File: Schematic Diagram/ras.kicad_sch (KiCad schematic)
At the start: 2 parts

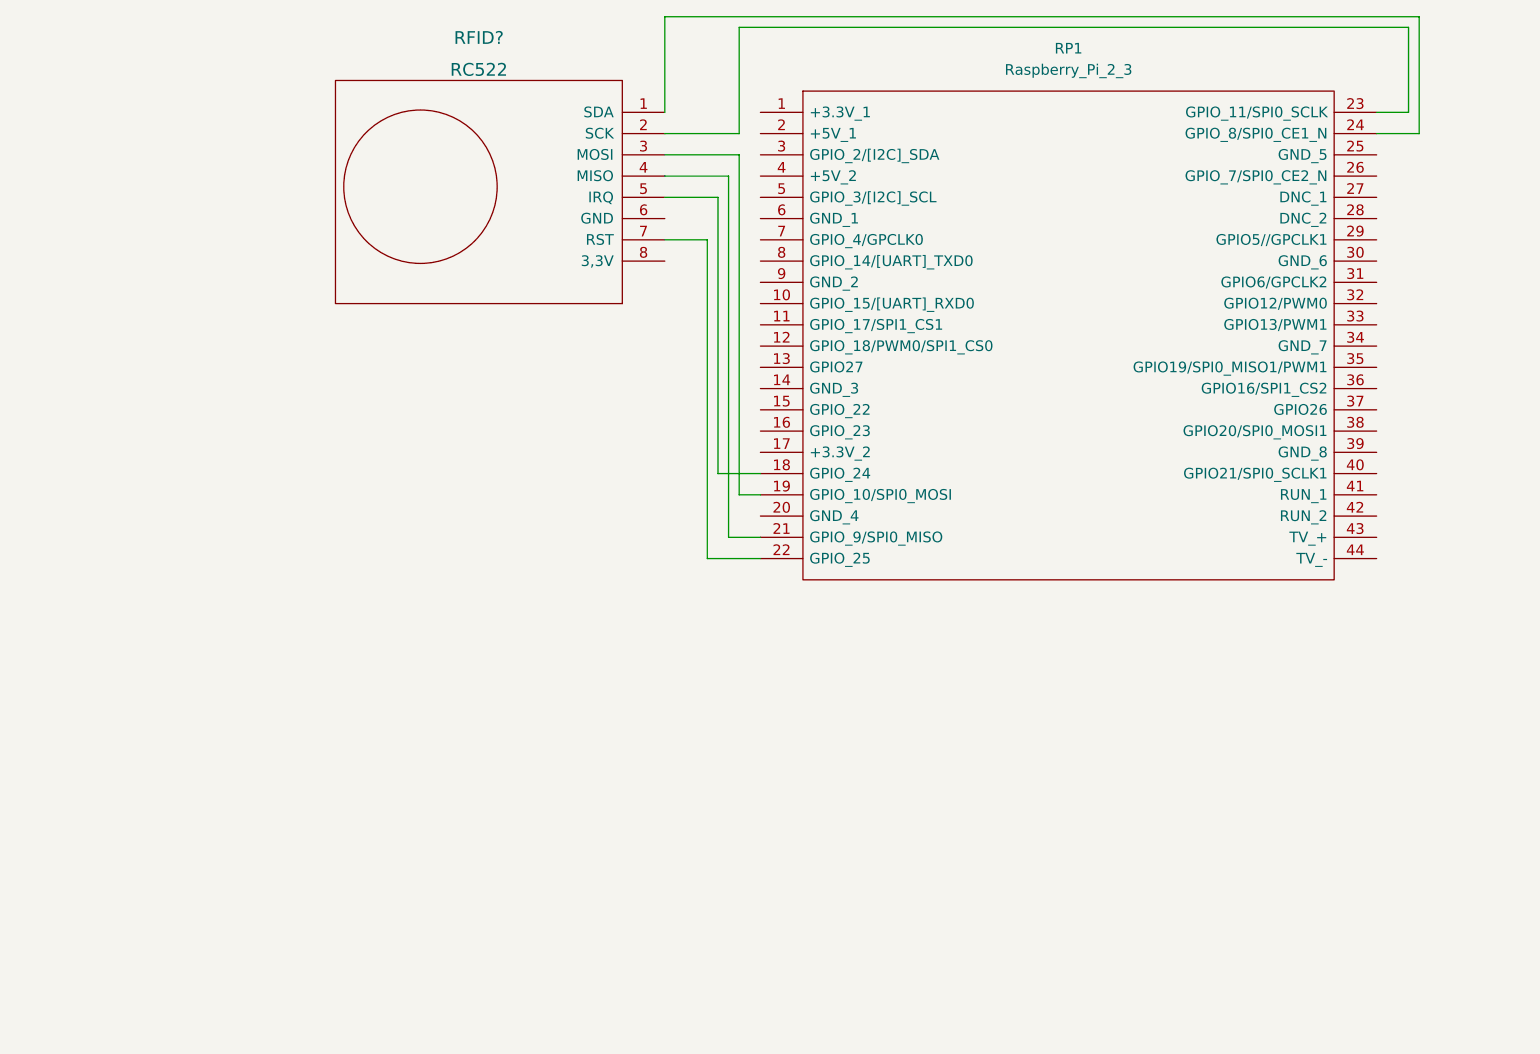
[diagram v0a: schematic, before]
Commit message: put RC522
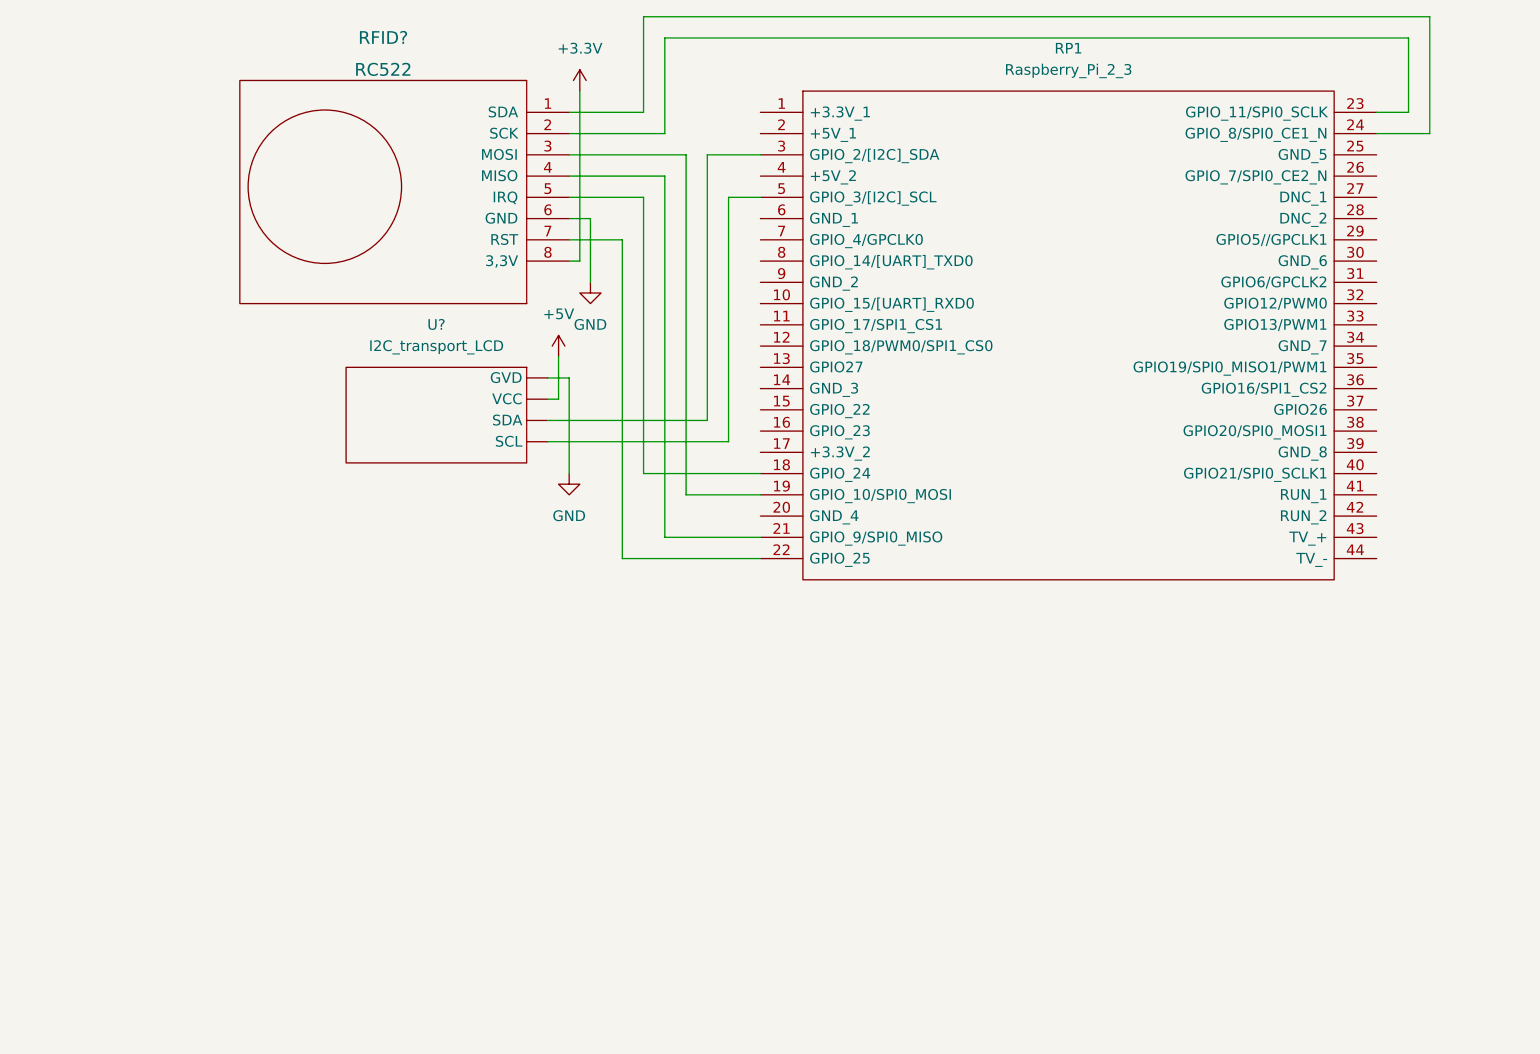
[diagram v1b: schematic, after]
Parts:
- added U?: I2C_transport_LCD, symbol project:I2C_transport_LCD
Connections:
- net at RP1.3 (GPIO_2/[I2C]_SDA): now also U?. (VCC)
- net at RP1.5 (GPIO_3/[I2C]_SCL): now also U?. (VCC)
- net GND: now reaches RFID?.6 (GND)
- net GND: now also U?. (VCC)
- net +3V3: now reaches RFID?.8 (3,3V)
- new net +5V: U?. (VCC)
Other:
- moved on the sheet: RFID?

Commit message: put LED
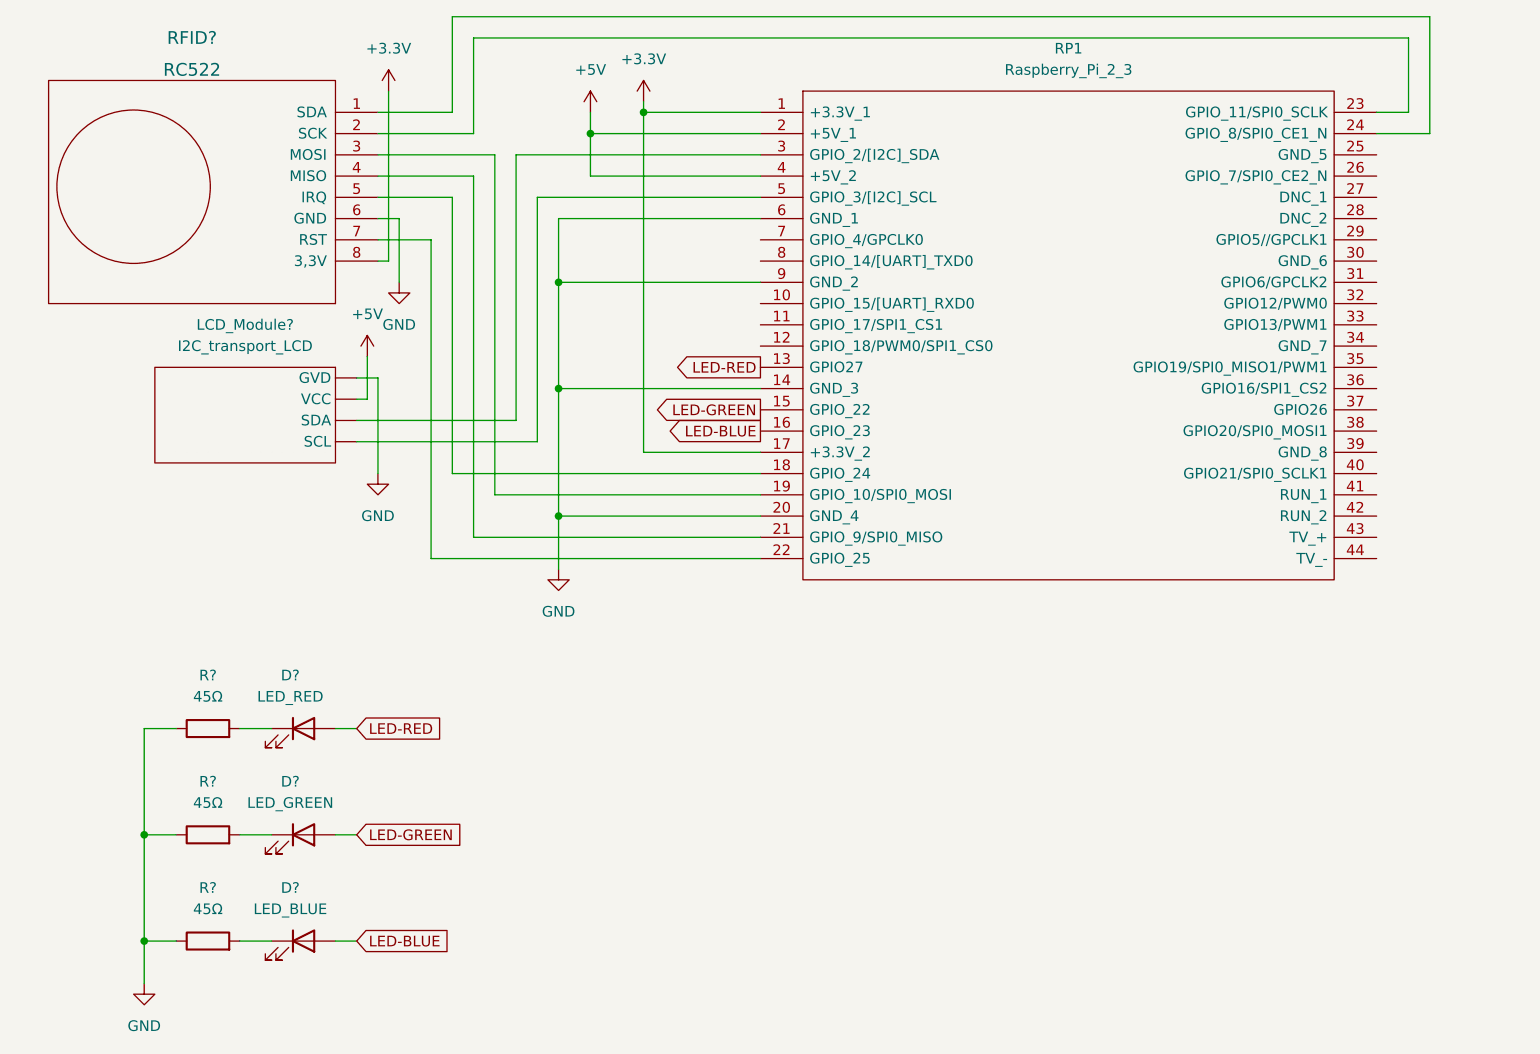
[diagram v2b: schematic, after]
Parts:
- removed U?: I2C_transport_LCD, symbol project:I2C_transport_LCD
- added D?: LED_RED, symbol Device:LED
- added D?: LED_GREEN, symbol Device:LED
- added D?: LED_BLUE, symbol Device:LED
- added LCD_Module?: I2C_transport_LCD, symbol project:I2C_transport_LCD
- added R? (x3): 45Ω, symbol Device:R
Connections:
- net +3V3: now also RP1.1 (+3.3V_1), RP1.17 (+3.3V_2)
- net +5V: now also RP1.2 (+5V_1), RP1.4 (+5V_2), LCD_Module?. (VCC)
- net GND: now also RP1.14 (GND_3), RP1.20 (GND_4), RP1.6 (GND_1), RP1.9 (GND_2), LCD_Module?. (VCC), R?.1, R?.1, R?.1
- net LED-RED: now reaches RP1.13 (GPIO27)
- net LED-RED: now also D?.2 (A)
- net LED-GREEN: now reaches RP1.15 (GPIO_22)
- net LED-GREEN: now also D?.2 (A)
- net LED-BLUE: now reaches RP1.16 (GPIO_23)
- net LED-BLUE: now also D?.2 (A)
- net at RP1.3 (GPIO_2/[I2C]_SDA): now also LCD_Module?. (VCC)
- net at RP1.5 (GPIO_3/[I2C]_SCL): now also LCD_Module?. (VCC)
- new net: D?.1 (K), R?.2 (x3)
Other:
- moved on the sheet: RFID?

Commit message: refactaring
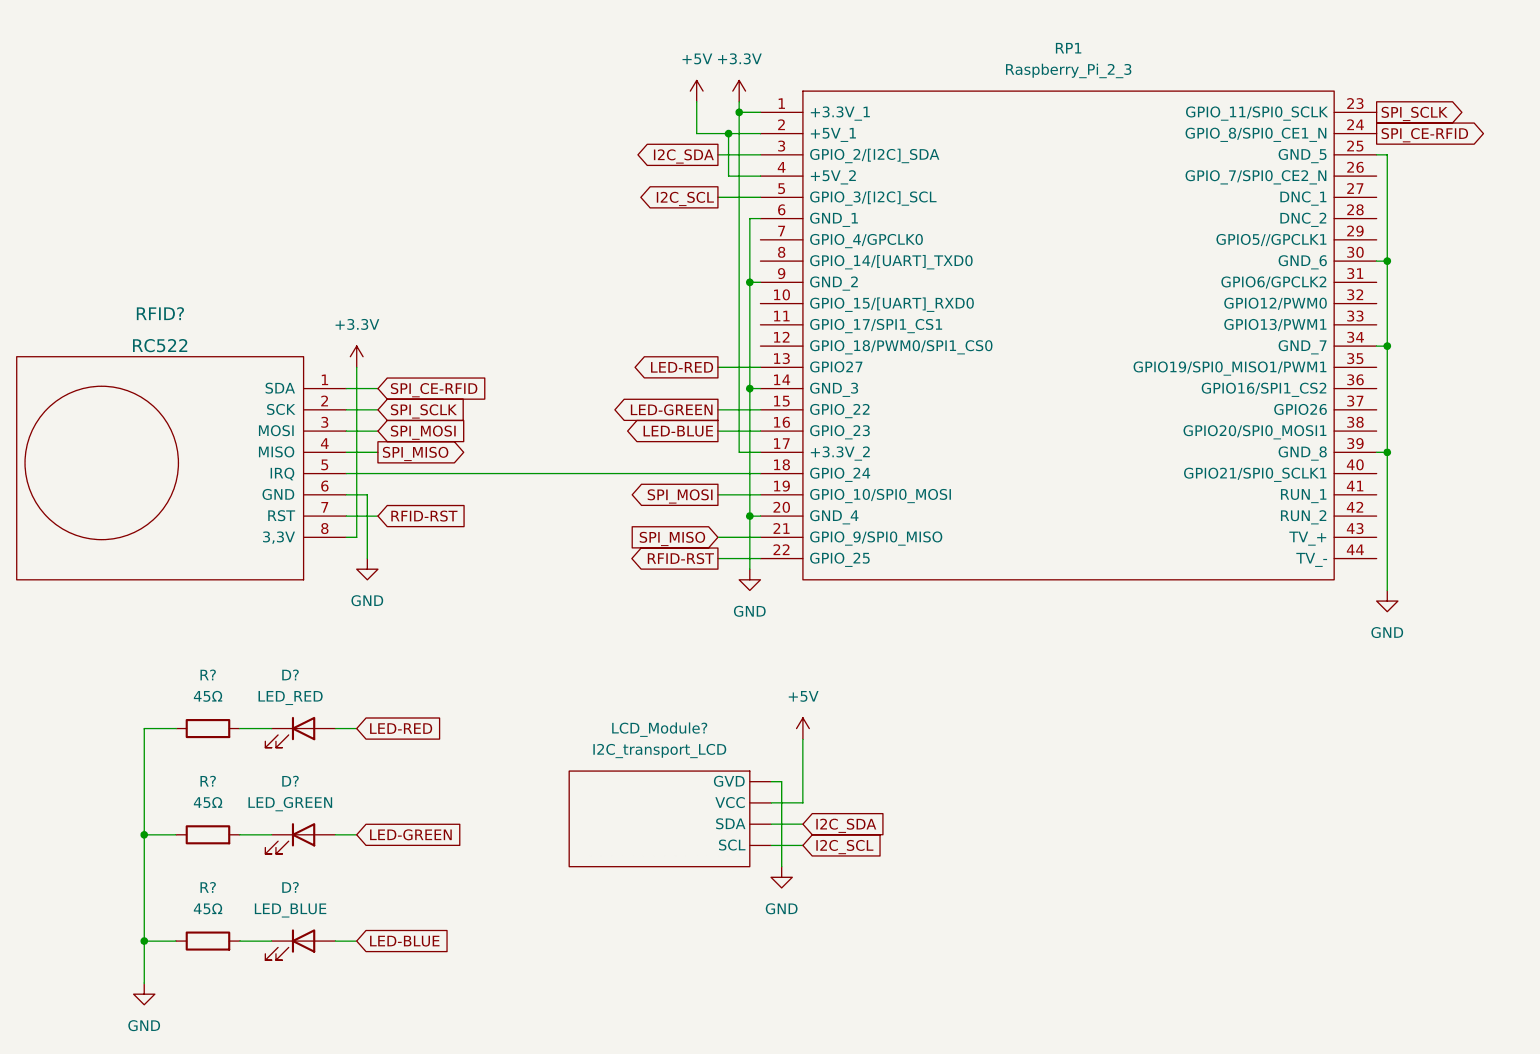
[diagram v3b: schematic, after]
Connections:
- net GND: now also RP1.25 (GND_5), RP1.30 (GND_6), RP1.34 (GND_7), RP1.39 (GND_8)
- net SPI_MOSI: now reaches RFID?.3 (MOSI), RP1.19 (GPIO_10/SPI0_MOSI)
- net SPI_MISO: now reaches RFID?.4 (MISO), RP1.21 (GPIO_9/SPI0_MISO)
- net RFID-RST: now reaches RFID?.7 (RST), RP1.22 (GPIO_25)
- net SPI_SCLK: now reaches RFID?.2 (SCK), RP1.23 (GPIO_11/SPI0_SCLK)
- net SPI_CE-RFID: now reaches RFID?.1 (SDA), RP1.24 (GPIO_8/SPI0_CE1_N)
- net I2C_SDA: now reaches LCD_Module?. (VCC), RP1.3 (GPIO_2/[I2C]_SDA)
- net I2C_SCL: now reaches LCD_Module?. (VCC), RP1.5 (GPIO_3/[I2C]_SCL)
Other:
- moved on the sheet: LCD_Module?, RFID?
